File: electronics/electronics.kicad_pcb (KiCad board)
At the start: 2 copper layers, 50.3 x 40.6 mm, 24 parts, among them J3 EXTERNAL CONTROL, J4 POWER, J5 I2C BUS, J6 I2C BUS, J7 INPUT, J8 OUTPUT, U1 ProMicro

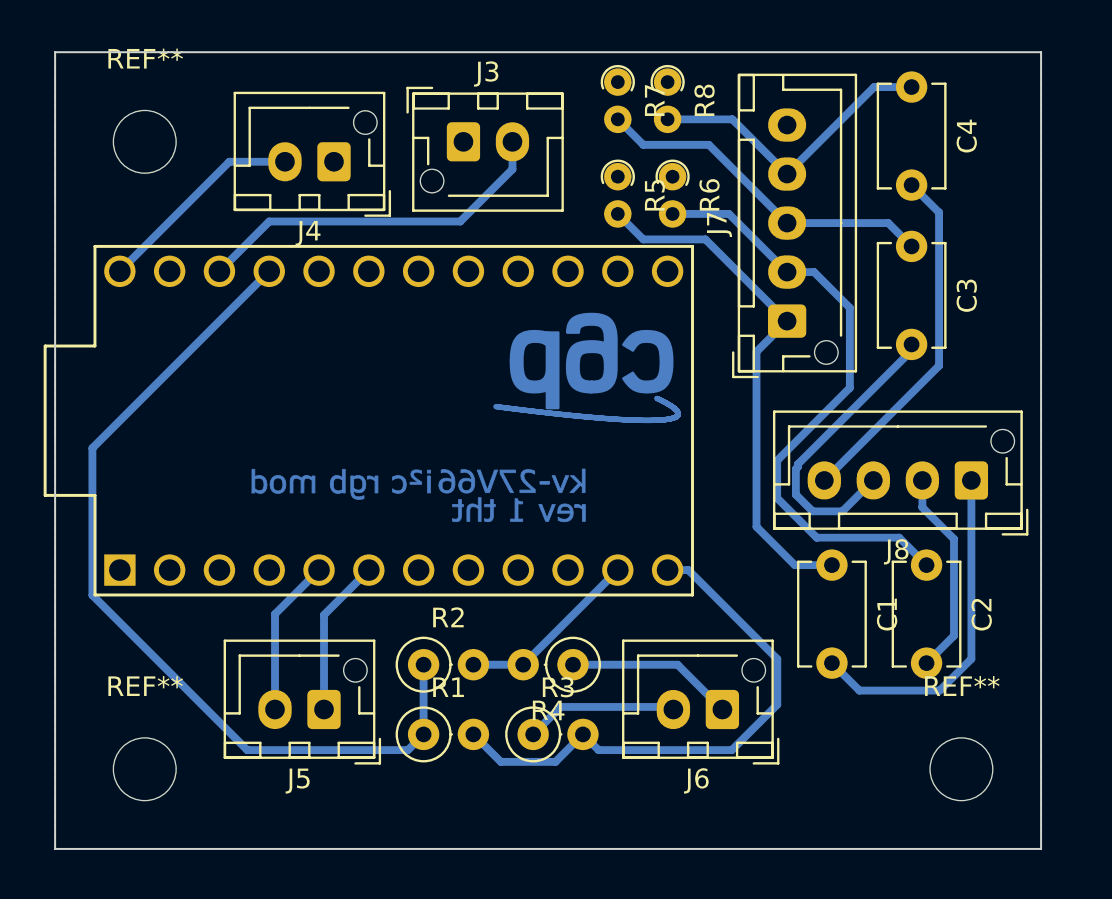
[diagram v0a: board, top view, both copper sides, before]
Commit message: Last through hole
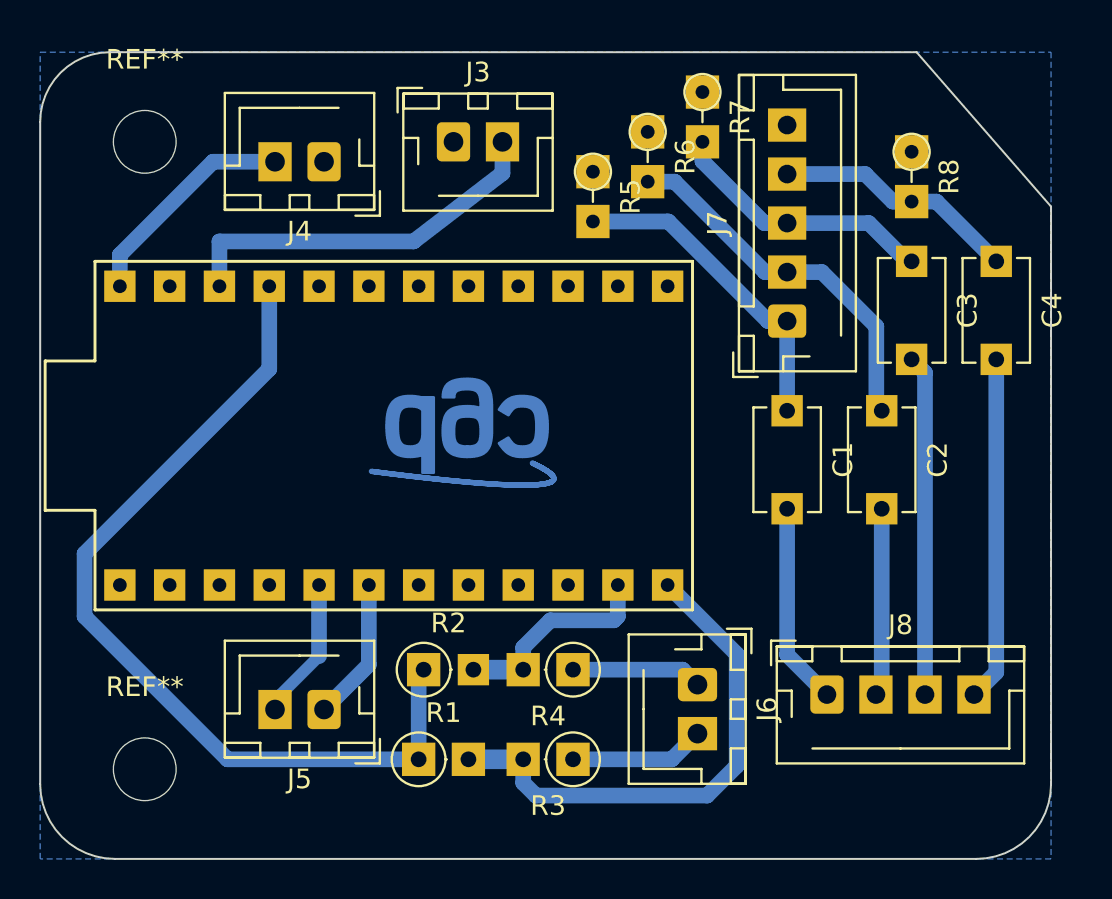
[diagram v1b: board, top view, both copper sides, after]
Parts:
- removed the REF** at (96.5, 54.4)
- removed the REF** at (138.2, 54.4)
- removed kv_revision: G***, local:kv27v66mod
- added REF**: MountingHole_3.2mm_M3_DIN965, MountingHole:MountingHole_3.2mm_M3_DIN965, F.Cu at (96.5, 54.4)
- R5, R6, R7, R8: footprint Resistor_THT:R_Axial_DIN0204_L3.6mm_D1.6mm_P1.90mm_Vertical -> Resistor_THT:R_Axial_DIN0204_L3.6mm_D1.6mm_P2.54mm_Vertical
- REF**: value MountingHole_3.2mm_M3 -> MountingHole_3.2mm_M3_DIN965; footprint MountingHole:MountingHole_3.2mm_M3 -> MountingHole:MountingHole_3.2mm_M3_DIN965
- moved J8 13.2 mm to (131.3, 50.5), turned to 0 degrees
- moved R8 12.9 mm to (135.6, 22.9)
- moved C4 9.88 mm to (140.0, 28.4)
- moved C1 8.20 mm to (129.3, 36.1)
- moved C2 8.20 mm to (134.1, 36.1)
- moved c6p_logo 7.16 mm to (113.8, 37.3)
- moved R7 4.35 mm to (125.0, 19.8)
- moved R6 2.62 mm to (122.2, 21.8)
- moved R3 2.40 mm to (118.4, 53.8), turned to 180 degrees
- moved J6 1.80 mm to (124.7, 50.0), turned to 270 degrees
- moved R5 1.30 mm to (119.4, 23.9)
- moved R1 1.30 mm to (110.5, 53.8)
- moved C3 0.76 mm to (135.6, 28.4)
- moved U1 0.76 mm to (109.2, 37.3)
- moved J3 0.51 mm to (112.3, 22.4)
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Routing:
- net GIN: track 31.3 -> 19.1 mm
- net RIN: track 26.7 -> 16.6 mm
- net ROUT: track 17.5 -> 10.3 mm
- net BIN: track 17.7 -> 13.8 mm
- net SYNCIN: track 15.4 -> 12.5 mm
- net BOUT: track 15.1 -> 17.4 mm
- net Net-(J6-Pad1): track 8.57 -> 6.67 mm
- net SCL2: track 9.36 -> 10.8 mm
- net RESET: track 18.5 -> 19.8 mm
- net SDA2: track 27.8 -> 26.5 mm
- net VCC: track 44.3 -> 45.5 mm
- net GOUT: track 10.6 -> 9.60 mm
- net Net-(J6-Pad2): track 7.79 -> 6.89 mm
- net SCL1: track 8.06 -> 7.30 mm
- net SDA1: track 8.04 -> 7.28 mm
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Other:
- board size 50.3 x 40.6 mm -> 51.6 x 41.1 mm
- net class Default: clearance 0.4 -> 0.6; trace_width 0.4 -> 0.8
- rule trace_clearance: 0.4 -> 0.6
